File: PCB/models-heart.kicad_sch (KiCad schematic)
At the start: 107 parts, among them P1 USB_C_Plug, Q1 AO3401A, Q2 FS8205, Q3 UMH3N, Q4 AO3401A, Q5 AO3401A, Q6 BC857BS, Q7 BC857BS, Q8 AO3401A, Q9 UMH3N, SW1 SW_Push, U1 TP4056, U2 DW01, U3 CH340C, U4 AMS1117-3.3, U5 ESP-12E, U6 DRV8833PWP

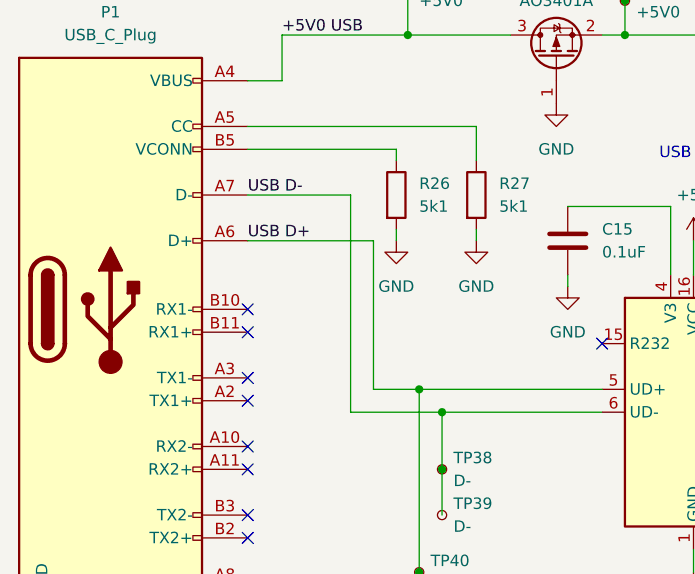
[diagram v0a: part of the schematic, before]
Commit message: actionns test
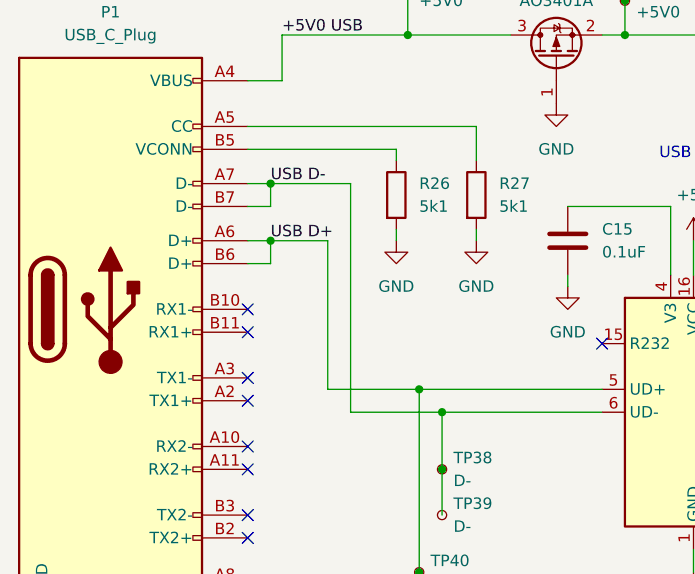
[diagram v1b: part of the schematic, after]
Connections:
- net USB D+: now also P1.B6 (D+)
- net USB D-: now also P1.B7 (D-)
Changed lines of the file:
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@@
   (junction (at 58.42 97.79) (diameter 0) (color 0 0 0 0)
   )
+  (junction (at 41.91 60.96) (diameter 0) (color 0 0 0 0)
+  )
   (junction (at 294.64 242.57) (diameter 0) (color 0 0 0 0)
   )
@@
   )
   (junction (at 368.3 168.91) (diameter 0) (color 0 0 0 0)
+  )
+  (junction (at 41.91 54.61) (diameter 0) (color 0 0 0 0)
   )
   (junction (at 199.39 130.81) (diameter 0) (color 0 0 0 0)
@@
     (stroke (width 0) (type default))
   )
+  (wire (pts (xy 39.37 57.15) (xy 41.91 57.15))
+    (stroke (width 0) (type default))
+  )
   (wire (pts (xy 142.24 242.57) (xy 144.78 242.57))
     (stroke (width 0) (type default))
@@
   )
   (wire (pts (xy 194.31 130.81) (xy 199.39 130.81))
+    (stroke (width 0) (type default))
+  )
+  (wire (pts (xy 41.91 60.96) (xy 39.37 60.96))
     (stroke (width 0) (type default))
   )
@@
     (stroke (width 0) (type default))
   )
+  (wire (pts (xy 41.91 54.61) (xy 39.37 54.61))
+    (stroke (width 0) (type default))
+  )
   (wire (pts (xy 114.3 124.46) (xy 114.3 129.54))
     (stroke (width 0) (type default))
@@
     (stroke (width 0) (type default))
   )
+  (wire (pts (xy 41.91 57.15) (xy 41.91 54.61))
+    (stroke (width 0) (type default))
+  )
   (wire (pts (xy 354.33 138.43) (xy 354.33 142.24))
     (stroke (width 0) (type default))
@@
     (stroke (width 0) (type default))
   )
+  (wire (pts (xy 41.91 60.96) (xy 48.26 60.96))
+    (stroke (width 0) (type default))
+  )
   (wire (pts (xy 64.77 52.07) (xy 64.77 48.26))
     (stroke (width 0) (type default))
@@
   )
   (wire (pts (xy 106.68 266.7) (xy 106.68 269.24))
-    (stroke (width 0) (type default))
-  )
-  (wire (pts (xy 39.37 55.88) (xy 50.8 55.88))
     (stroke (width 0) (type default))
   )
@@
     (stroke (width 0) (type default))
   )
+  (wire (pts (xy 41.91 63.5) (xy 41.91 60.96))
+    (stroke (width 0) (type default))
+  )
   (wire (pts (xy 259.08 245.11) (xy 260.35 245.11))
     (stroke (width 0) (type default))
@@
     (stroke (width 0) (type default))
   )
-  (wire (pts (xy 39.37 60.96) (xy 53.34 60.96))
-    (stroke (width 0) (type default))
-  )
   (wire (pts (xy 252.73 142.24) (xy 254 142.24))
     (stroke (width 0) (type default))
@@
     (stroke (width 0) (type default))
   )
-  (wire (pts (xy 53.34 60.96) (xy 53.34 77.47))
+  (wire (pts (xy 48.26 60.96) (xy 48.26 77.47))
     (stroke (width 0) (type default))
   )
@@
     (stroke (width 0) (type default))
   )
-  (wire (pts (xy 53.34 77.47) (xy 58.42 77.47))
+  (wire (pts (xy 48.26 77.47) (xy 58.42 77.47))
     (stroke (width 0) (type default))
   )
@@
     (stroke (width 0) (type default))
   )
-  (wire (pts (xy 50.8 55.88) (xy 50.8 80.01))
+  (wire (pts (xy 50.8 54.61) (xy 50.8 80.01))
     (stroke (width 0) (type default))
   )
@@
   )
   (wire (pts (xy 151.13 250.19) (xy 151.13 245.11))
+    (stroke (width 0) (type default))
+  )
+  (wire (pts (xy 41.91 54.61) (xy 50.8 54.61))
     (stroke (width 0) (type default))
   )
@@
     (stroke (width 0) (type default))
   )
+  (wire (pts (xy 39.37 63.5) (xy 41.91 63.5))
+    (stroke (width 0) (type default))
+  )
   (wire (pts (xy 242.57 78.74) (xy 242.57 82.55))
     (stroke (width 0) (type default))
@@
     (effects (font (size 1.27 1.27)) (justify left bottom))
   )
-  (label "USB D+" (at 39.37 60.96 0) (fields_autoplaced)
-    (effects (font (size 1.27 1.27)) (justify left bottom))
-  )
-  (label "USB D-" (at 39.37 55.88 0) (fields_autoplaced)
+  (label "USB D+" (at 41.91 60.96 0) (fields_autoplaced)
+    (effects (font (size 1.27 1.27)) (justify left bottom))
+  )
+  (label "USB D-" (at 41.91 54.61 0) (fields_autoplaced)
     (effects (font (size 1.27 1.27)) (justify left bottom))
   )
@@
     (pin "A5")
     (pin "A6")
+    (pin "B6")
     (pin "A7")
+    (pin "B7")
     (pin "A8")
     (pin "A9")
